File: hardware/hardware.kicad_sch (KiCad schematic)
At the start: 0 parts

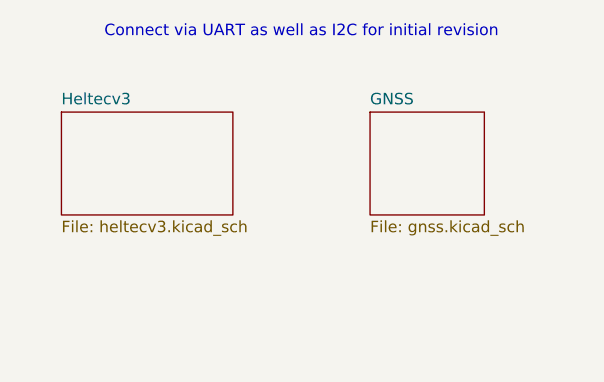
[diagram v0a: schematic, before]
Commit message: Prel. pin assignments for base station
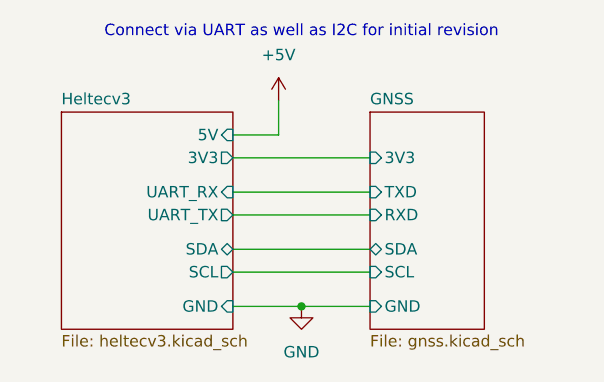
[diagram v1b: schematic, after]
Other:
- sheet GNSS ports: added 3V3, GND, RXD, SCL, SDA, TXD; removed none
- sheet Heltecv3 ports: added 3V3, 5V, GND, SCL, SDA, UART_RX, UART_TX; removed none
